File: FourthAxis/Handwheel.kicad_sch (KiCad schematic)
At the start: 5 parts, among them U5 LMV393

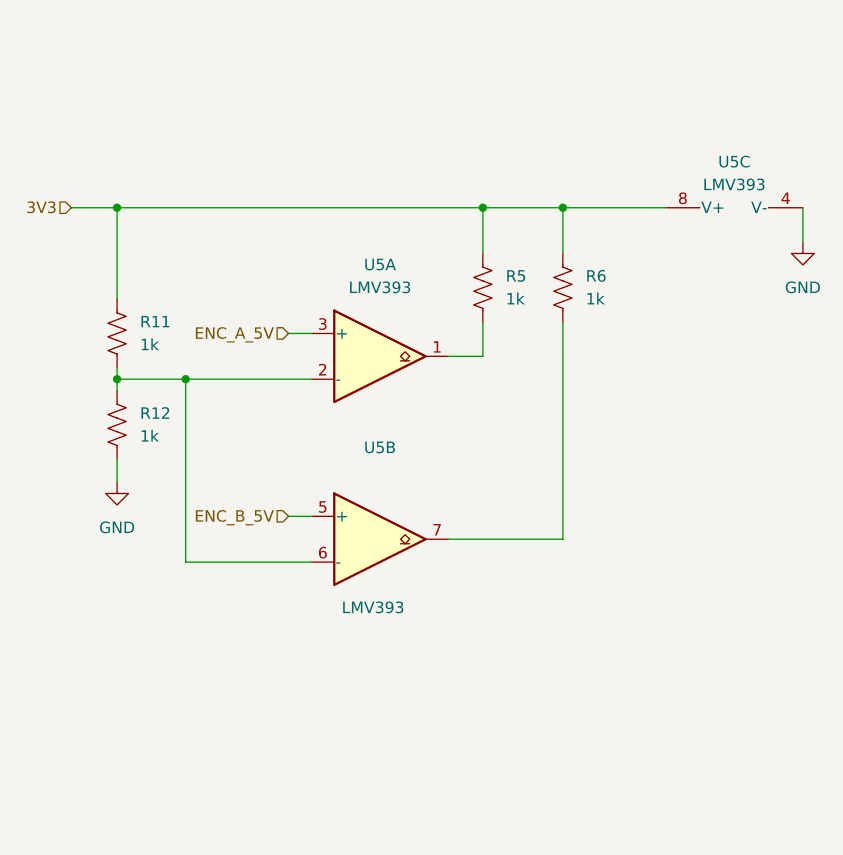
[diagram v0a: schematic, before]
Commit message: schem additions
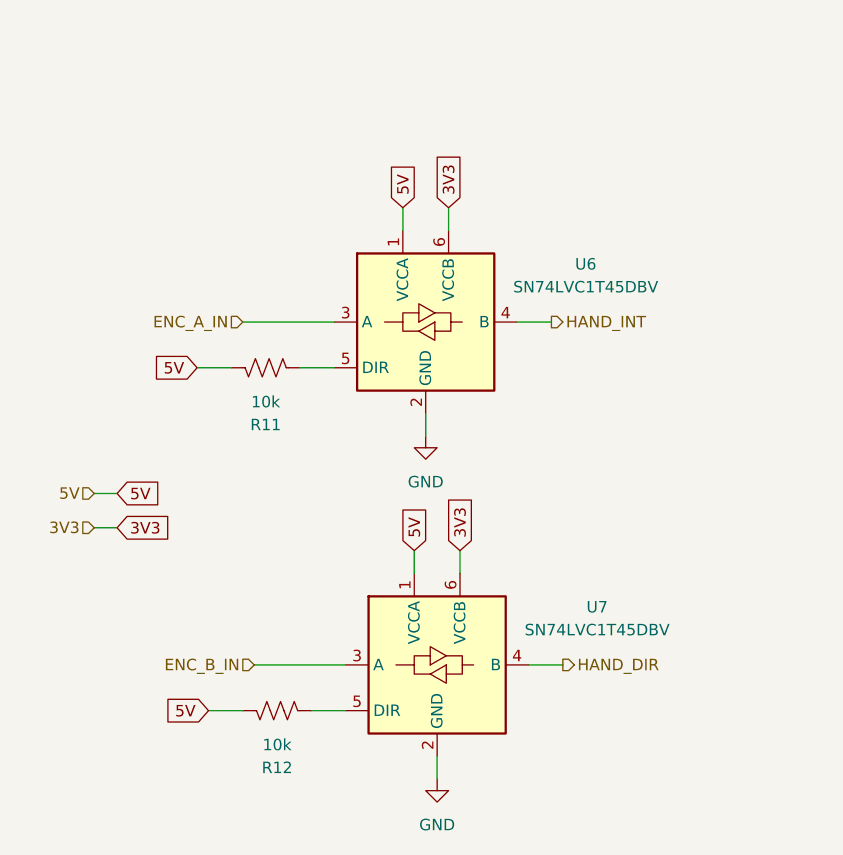
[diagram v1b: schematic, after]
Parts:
- removed R5, R6: 1k, symbol Device:R_US
- removed U5: LMV393, symbol Comparator:LMV393
- added U6, U7: SN74LVC1T45DBV, Package_TO_SOT_SMD:SOT-23-6, symbol Logic_LevelTranslator:SN74LVC1T45DBV
- R11, R12: value 1k -> 10k
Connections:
- net 3V3: now also U6.6 (VCCB), U7.6 (VCCB); no longer R11.1
- net GND: now also U6.2 (GND), U7.2 (GND); no longer R12.2
- net at R11.2: now also U6.5 (DIR); no longer R12.1
- new net: R12.2, U7.5 (DIR)
- new net 5V: R11.1, R12.1, U6.1 (VCCA), U7.1 (VCCA)
- new net ENC_A_IN: U6.3 (A)
- new net ENC_B_IN: U7.3 (A)
- new net HAND_DIR: U7.4 (B)
- new net HAND_INT: U6.4 (B)

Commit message: name and layout
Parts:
- R11, R12: footprint (none) -> Resistor_SMD:R_0603_1608Metric
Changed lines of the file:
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@@
 			)
 		)
-		(property "Footprint" ""
+		(property "Footprint" "Resistor_SMD:R_0603_1608Metric"
 			(at 68.834 97.536 90)
 			(hide yes)
@@
 			)
 		)
-		(property "Footprint" ""
+		(property "Footprint" "Resistor_SMD:R_0603_1608Metric"
 			(at 67.564 59.436 90)
 			(hide yes)

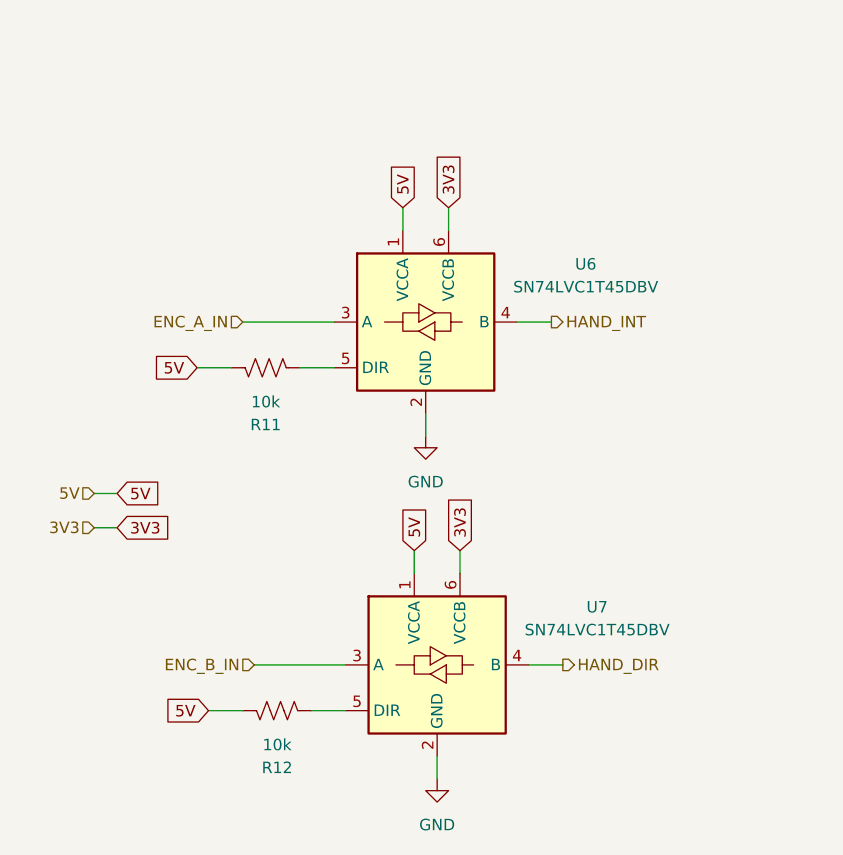
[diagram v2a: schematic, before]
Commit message: Nick end of wed
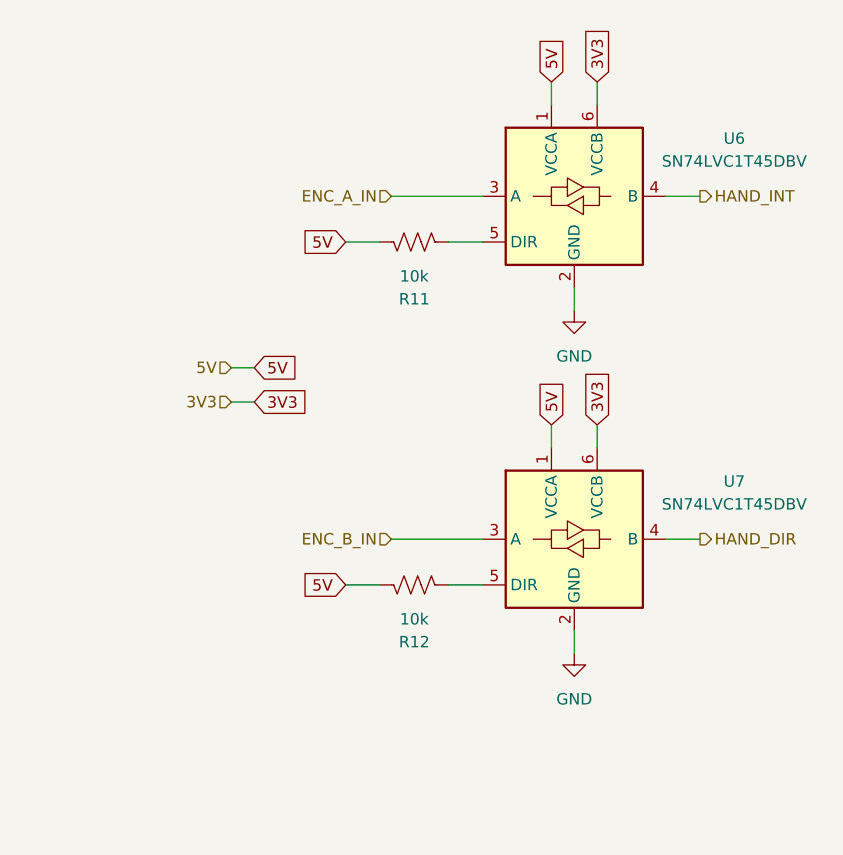
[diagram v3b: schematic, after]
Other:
- moved on the sheet: R11, R12, U6, U7
